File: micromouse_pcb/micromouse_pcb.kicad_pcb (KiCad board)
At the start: 2 copper layers, 106.5 x 143.3 mm, 55 parts, among them J103 Conn_01x10, J104 Conn_01x02, J105 Conn_01x06, J106 Conn_01x02, J111 Conn_01x06, Q101 BS170, Q102 SFH313FA, Q103 SFH313FA, Q104 SFH313FA, Q105 SFH313FA, Q106 BS170, Q107 BS170, Q108 BS170, U103 L293D, U104 Teensy4.1_bare, U105 MCP3004

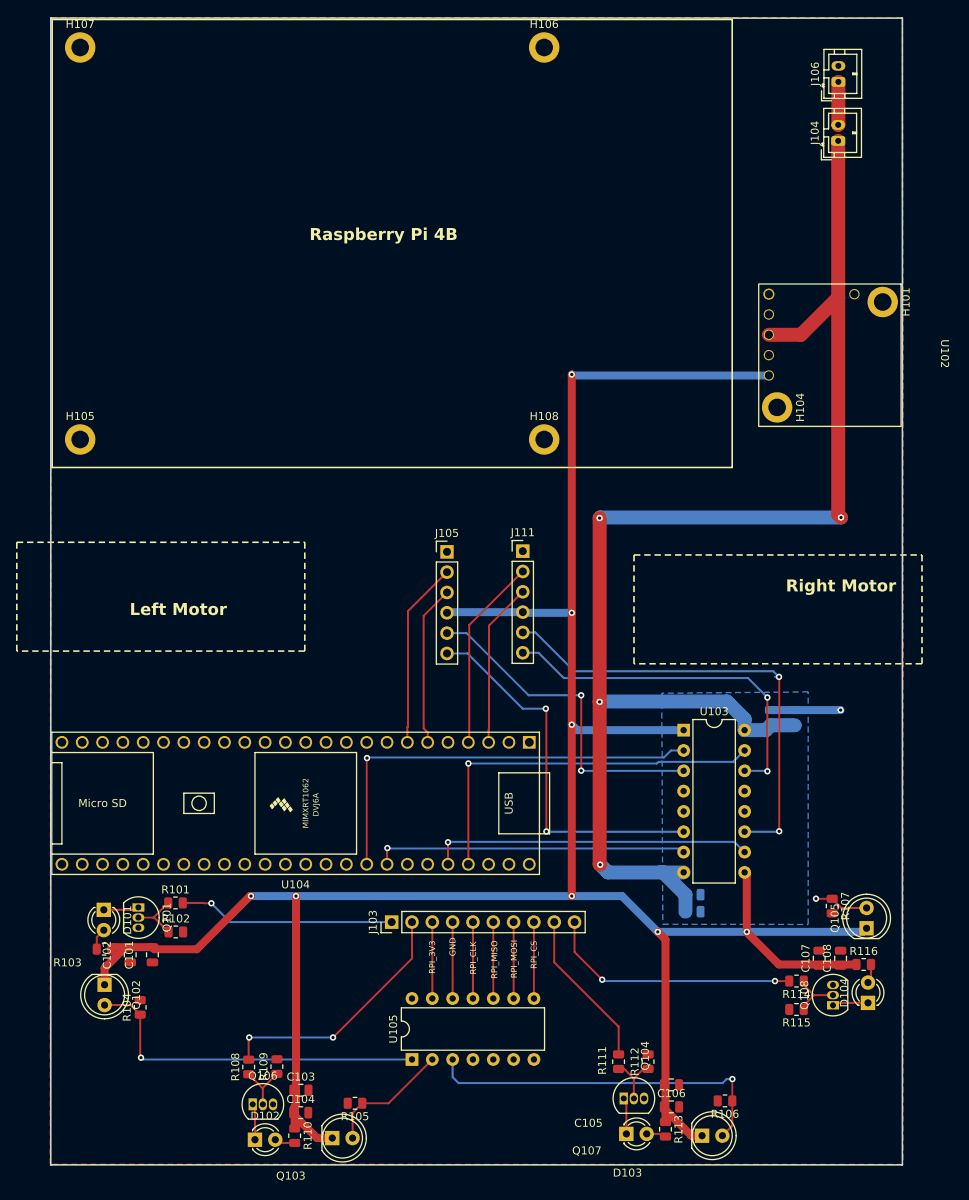
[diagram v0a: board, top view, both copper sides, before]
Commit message: updated pcb
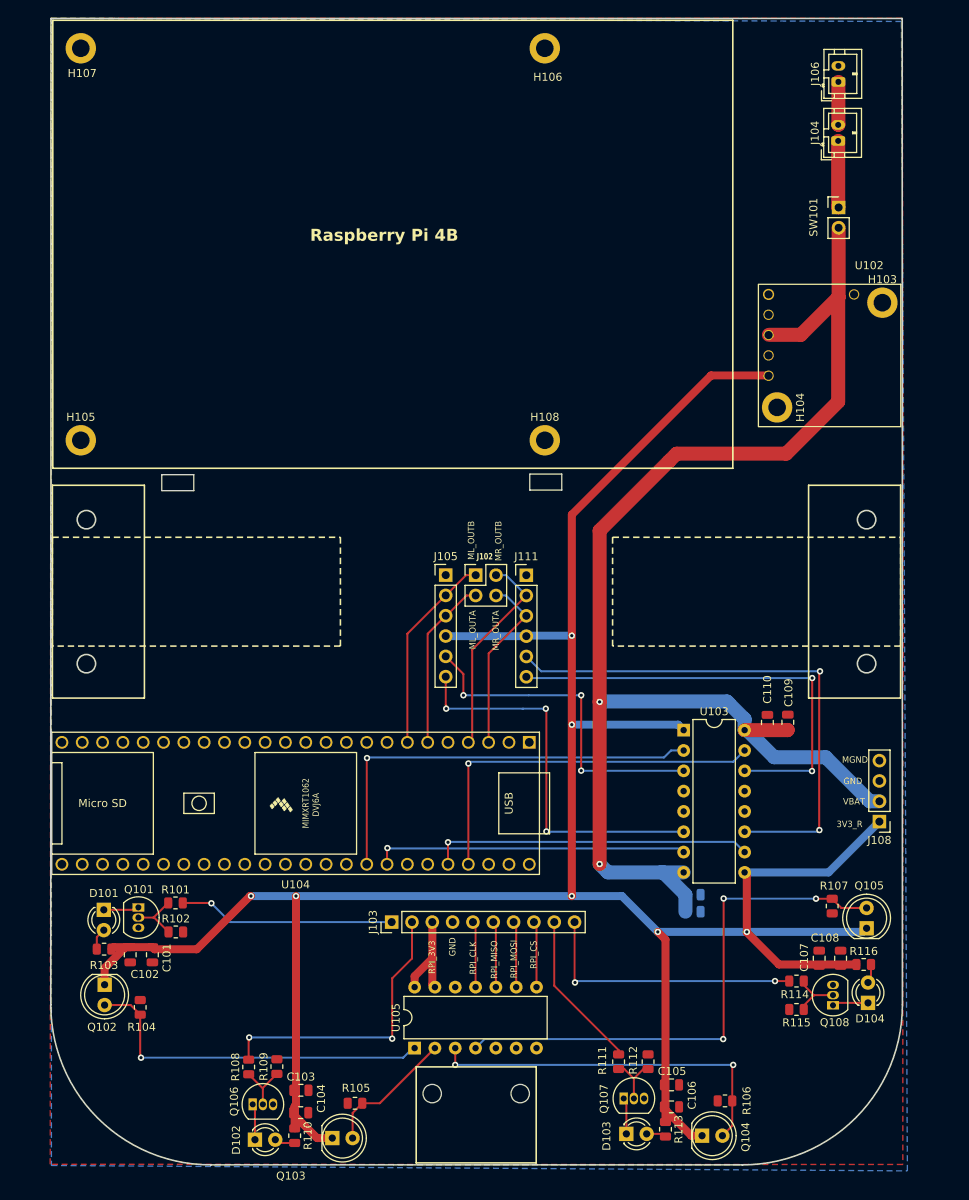
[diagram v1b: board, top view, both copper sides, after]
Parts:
- removed H101: MountingHole_Pad, MountingHole:MountingHole_2.2mm_M2_DIN965_Pad
- added H103: MountingHole_Pad, MountingHole:MountingHole_2.2mm_M2_DIN965_Pad, F.Cu at (156.6, 58.2)
- added J102: Conn_02x02_Counter_Clockwise, Connector_PinHeader_2.54mm:PinHeader_2x02_P2.54mm_Vertical, F.Cu at (105.8, 92.3)
- added J108: Conn_01x04, Connector_PinHeader_2.54mm:PinHeader_1x04_P2.54mm_Vertical, F.Cu at (156.2, 123.1)
- added SW101: SW_SPST, Connector_PinHeader_2.54mm:PinHeader_1x02_P2.54mm_Vertical, F.Cu at (151.2, 46.4)
- C109, C110: moved to F.Cu
- R103: value 50 Ohm -> 51Ohm
- R110, R113: value 50 Ohm -> 51 Ohm
- moved J111 3.04 mm to (112.1, 92.3)
- moved J105 2.91 mm to (102.0, 92.3)
- moved U105 1.46 mm to (98.2, 151.4)
- moved C109 1.05 mm to (144.8, 110.7)
- moved C110 0.73 mm to (142.2, 110.7)
- moved H108 0.13 mm to (114.4, 75.5)
- moved H105 0.13 mm to (56.4, 75.5)
- moved H106 0.12 mm to (114.4, 26.4)
- moved H107 0.12 mm to (56.4, 26.4)
- moved U102 0.05 mm to (160.5, 61.5)
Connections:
- J104 pad 1: /VBAT -> Net-(J104-Pin_1)
- U104 pad 15: /TEENSY_3V3 -> unconnected-(U104-3V3-Pad15)
- U104 pad 46: /TEENSY_3V3 -> unconnected-(U104-3V3-Pad46)
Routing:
- net /IR_RECEIVER_4: track 6.81 -> 67.4 mm, vias 1 -> 3
- net GND: track 18.3 -> 0.00 mm, vias 1 -> 0
- net /MR_1: track 45.0 -> 55.9 mm
- net /3V3_REGULATED: track 315.5 -> 324.7 mm, vias 8 -> 7
- net Net-(J104-Pin_1): track 0.00 -> 8.35 mm
- net /MR_2: track 58.5 -> 66.8 mm
- net /IR_EMITTER_2: track 31.8 -> 36.3 mm
- net /RPI_3V3: track 9.55 -> 13.2 mm
- net /MR_OUTA: track 20.6 -> 23.3 mm
- net /IR_EMITTER_4: track 32.1 -> 34.4 mm
- net /MR_OUTB: track 24.2 -> 26.2 mm
- net /ML_OUTB: track 23.3 -> 25.1 mm
- net /ML_OUTA: track 20.2 -> 21.6 mm
- net /VBAT: track 175.7 -> 174.4 mm, vias 4 -> 2
- net /RPI_MOSI: track 9.55 -> 8.26 mm
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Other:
- outline, holes or cut-outs redrawn
- board text added: "3V3_R"
- board text added: "Adam Casselman Arna Bharadwaj Siddhant Panse"
- board text added: "MGND"
- board text added: "ML_OUTA"
- board text added: "ML_OUTB"
- board text added: "MR_OUTA"
- board text added: "MR_OUTB"
- board text added: "VBAT"
- board text removed: "Left Motor"
- board text removed: "Right Motor"
